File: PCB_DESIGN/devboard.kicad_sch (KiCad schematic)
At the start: 33 parts, among them J1 USB_C_Receptacle_USB2.0_14P, J2 Conn_01x20, J3 Conn_01x20, J4 Conn_01x03, SW1 SW_Push, U1 RP2040, U2 NCP1117-3.3_SOT223, U3 W25Q128JVS, Y1 12 MHz

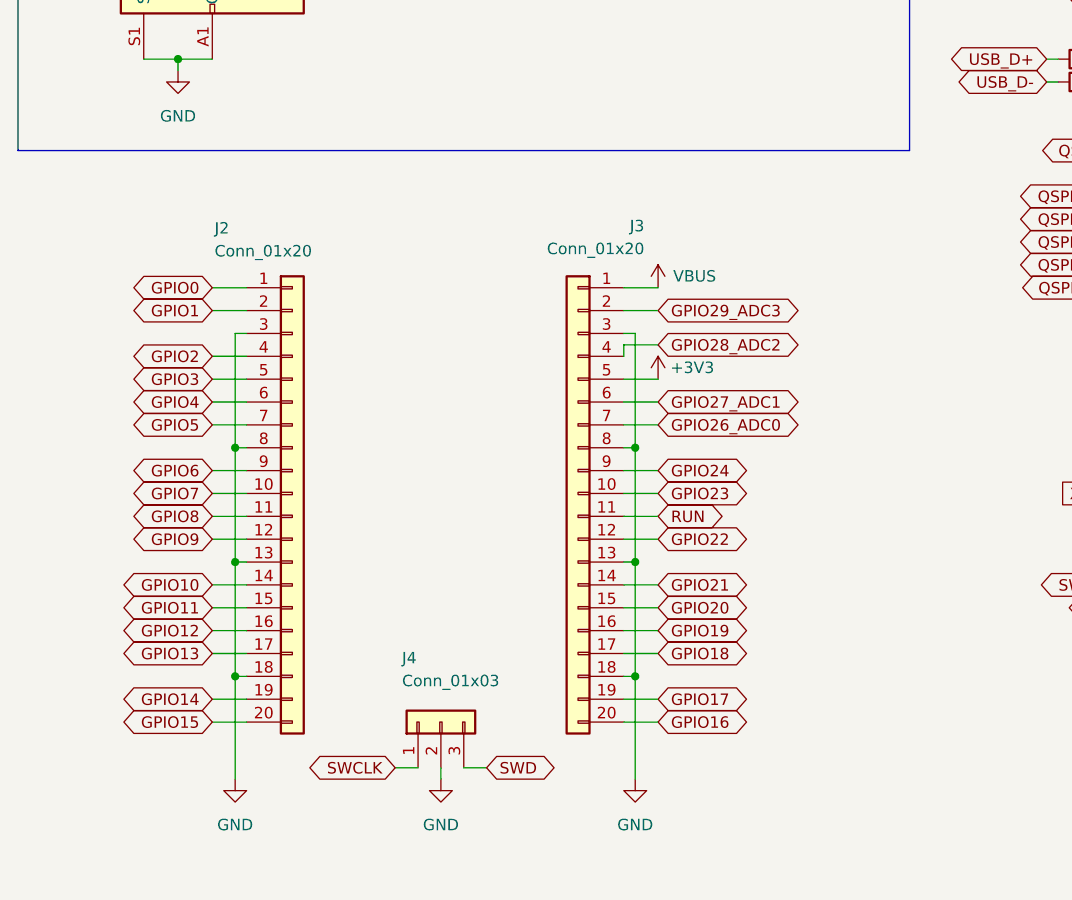
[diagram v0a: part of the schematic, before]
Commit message: assigned new footpritns and updating journal
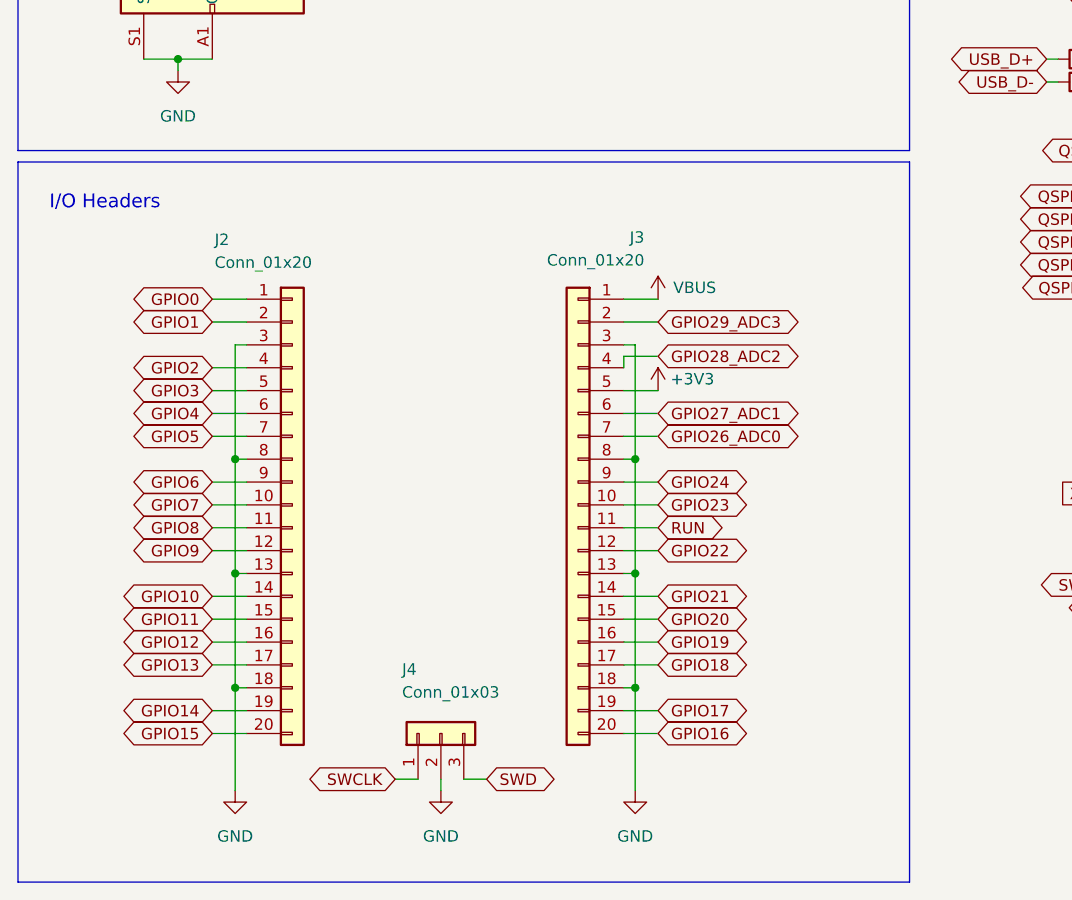
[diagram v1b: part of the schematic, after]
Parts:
- J2, J3: footprint (none) -> Connector_PinHeader_2.54mm:PinHeader_1x20_P2.54mm_Vertical
- J4: footprint (none) -> Connector_PinHeader_2.54mm:PinHeader_1x03_P2.54mm_Vertical
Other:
- note added: "I/O Headers"
- moved on the sheet: J2, J3, J4
